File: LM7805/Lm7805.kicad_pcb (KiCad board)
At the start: 2 copper layers, 34.5 x 34 mm, 9 parts, among them P1 CONN_02X04, P2 CONN_01X03, P3 CONN_01X03, P4 CONN_01X03, U1 LM7805CT

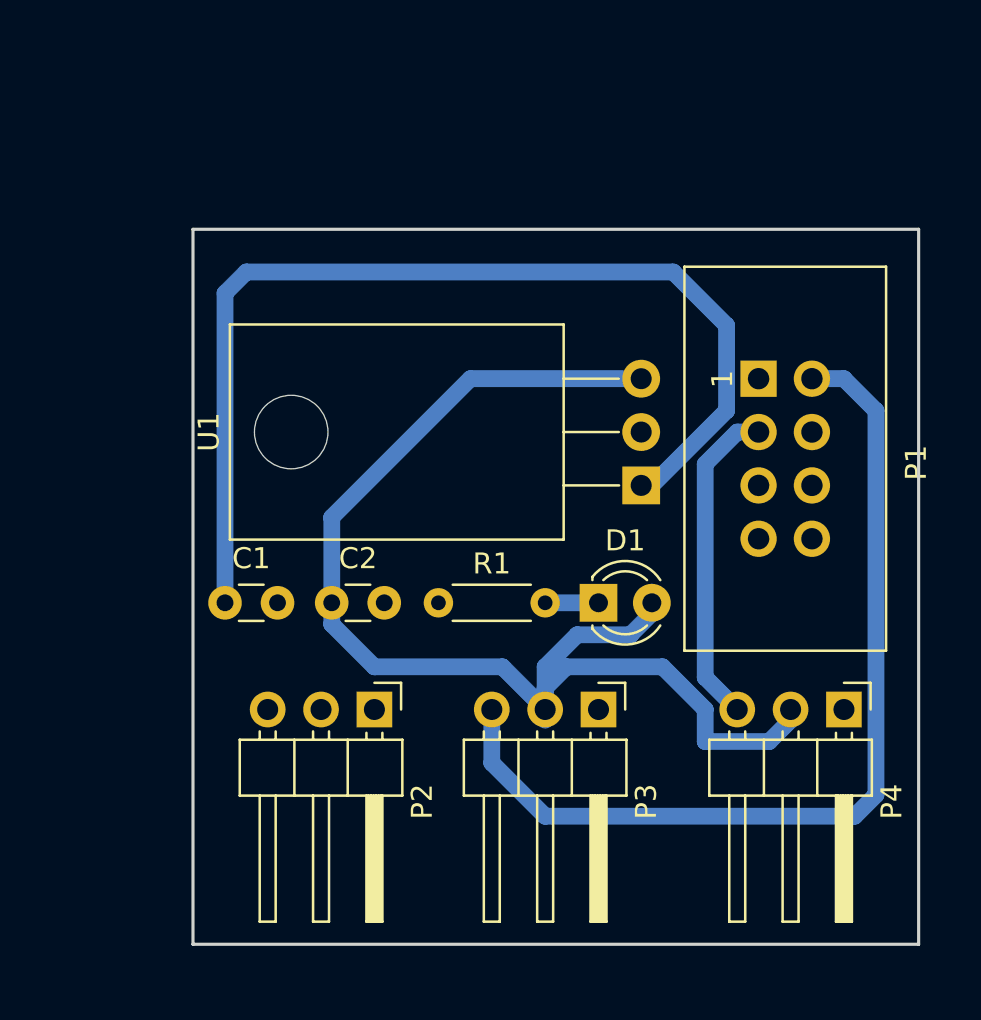
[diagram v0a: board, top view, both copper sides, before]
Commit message: final pcb
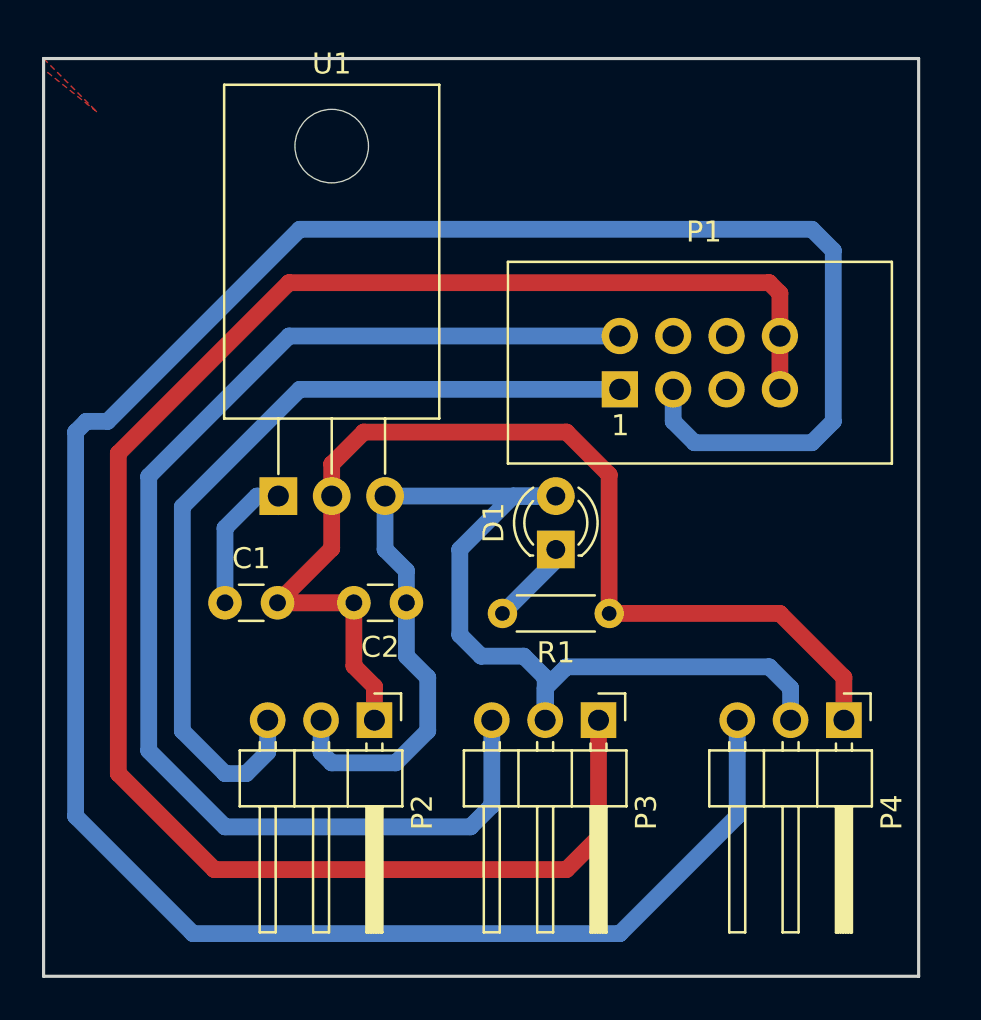
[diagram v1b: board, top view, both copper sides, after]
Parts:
- moved U1 17.3 mm to (136.1, 114.3), turned to 0 degrees
- moved R1 8.14 mm to (151.9, 119.9), turned to 180 degrees
- moved P1 6.62 mm to (152.4, 109.2), turned to 0 degrees
- moved C2 3.56 mm to (142.2, 119.4), turned to 180 degrees
- moved D1 3.25 mm to (149.4, 116.8), turned to 90 degrees
- moved P2 0.51 mm to (140.7, 125.0)
- moved P3 0.51 mm to (151.4, 125.0)
- moved P4 0.51 mm to (163.1, 125.0)
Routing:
- net GND: track 0.00 -> 138.9 mm
- net /PD13: track 15.5 -> 117.6 mm
- net +BATT: track 49.7 -> 7.24 mm
- net /PD11: track 0.00 -> 40.7 mm
- net /PD12: track 44.3 -> 60.6 mm
- net Net-(D1-Pad1): track 2.54 -> 4.10 mm
- added copper zone on F.Cu, net GND
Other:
- board size 34.5 x 34 mm -> 41.7 x 43.7 mm
- net class Default: clearance 0.2 -> 0.8
- rule trace_clearance: 0.2 -> 0.8
